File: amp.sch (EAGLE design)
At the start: 2 parts

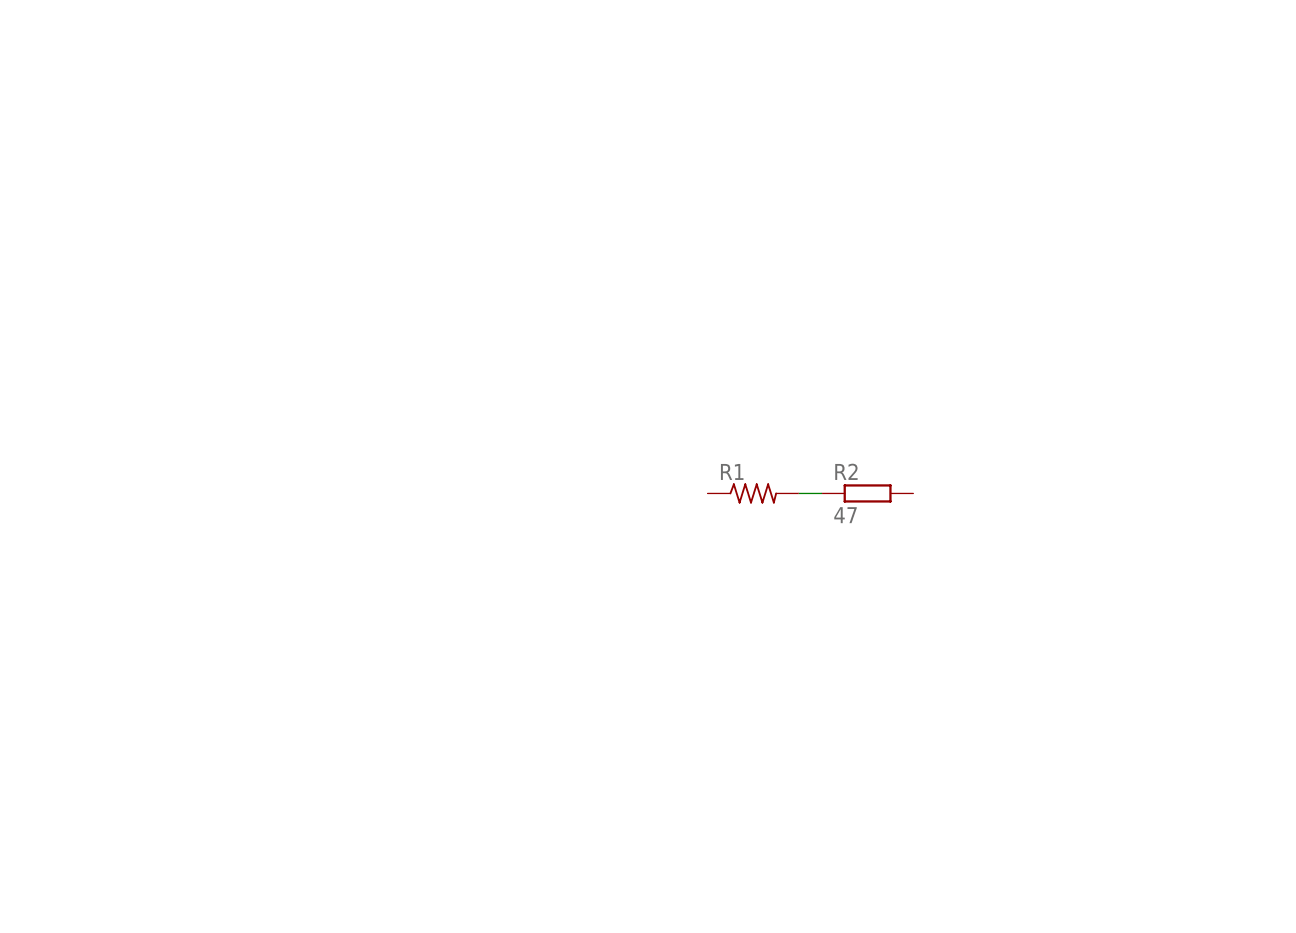
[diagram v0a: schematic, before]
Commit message: emmegmi
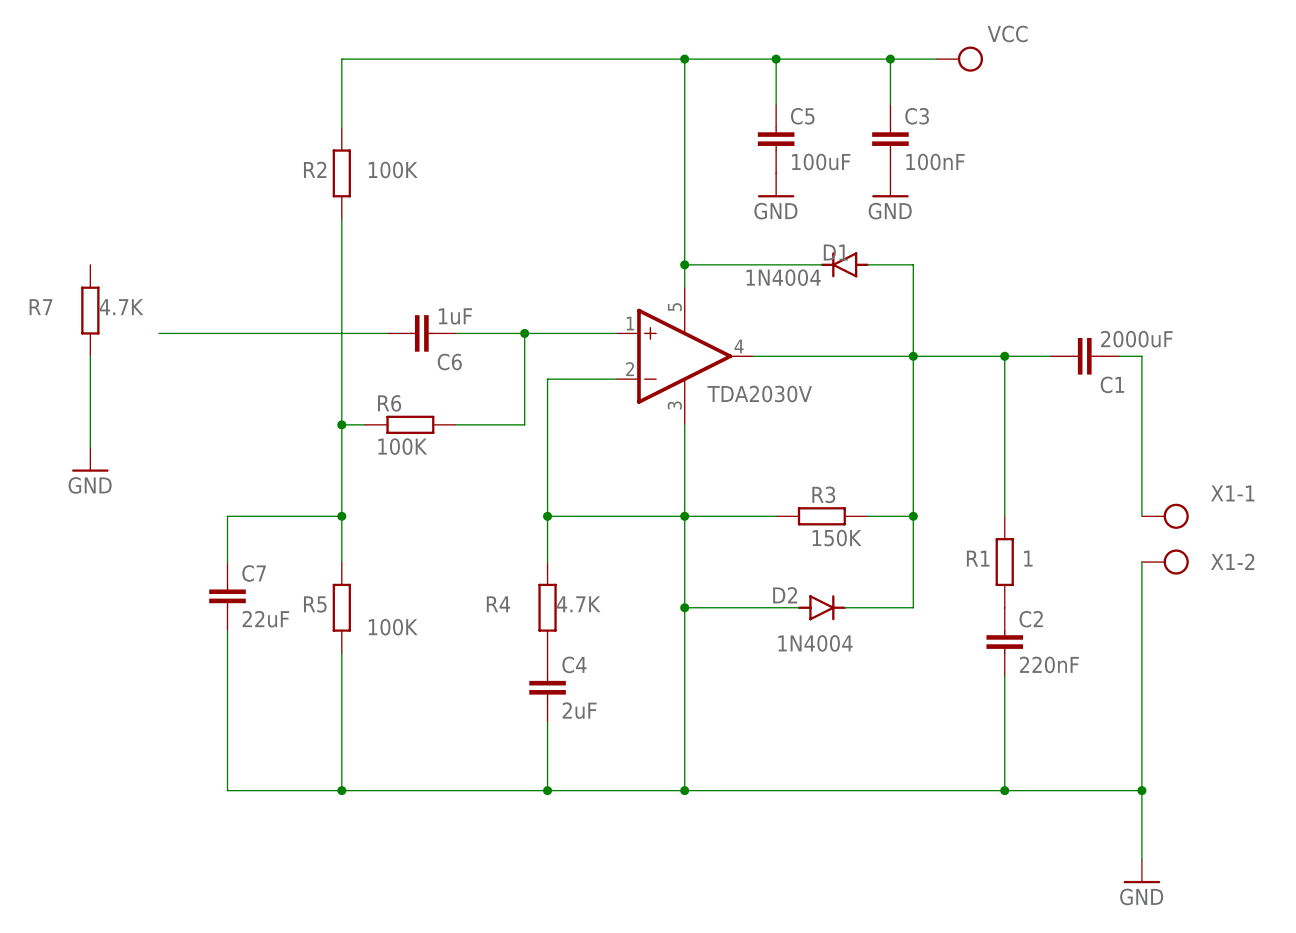
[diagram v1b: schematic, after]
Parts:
- added C1: 2000uF, capacitor-wima:C2,5-3
- added C2: 220nF, capacitor-wima:C2,5-3
- added C3: 100nF, capacitor-wima:C2,5-3
- added C4: 2uF, capacitor-wima:C2,5-3
- added C5: 100uF, capacitor-wima:C2,5-3
- added C6: 1uF, capacitor-wima:C2,5-3
- added C7: 22uF, capacitor-wima:C2,5-3
- added D1, D2: 1N4004, diode:1N4004
- added IC1: TDA2030V, linear:TDA2030V
- added R3: 150K, rcl:R-EU_0207/12
- added R4, R7: 4.7K, rcl:R-EU_0207/12
- added R5, R6: 100K, rcl:R-EU_0207/12
- added X1: (no value), con-wago-500:W237-113
- R1: value (none) -> 1; device rcl:R-US_0207/15 -> rcl:R-EU_0207/12
- R2: value 47 -> 100K
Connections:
- new net GND: C2.2, C3.2, C4.2, C5.2, C7.2, D2.A, IC1.-IN, IC1.GND, R3.1, R4.2, R5.1, R7.1, X1-2.KL
- new net N$2: C1.1, X1-1.KL
- new net N$3: C6.1, IC1.+IN, R6.2
- new net N$4: C1.2, D1.A, D2.C, IC1.OUT, R1.2, R3.2
- new net N$5: C2.1, R1.1
- new net N$6: C7.1, R2.1, R5.2, R6.1
- new net N$9: C6.2
- new net VCC: C3.1, C5.1, D1.C, IC1.V+, R2.2
- net N$1: now also C4.1, R4.1; no longer R1.2, R2.1
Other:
- moved on the sheet: R2
